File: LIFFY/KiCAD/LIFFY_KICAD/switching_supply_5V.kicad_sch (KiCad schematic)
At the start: 6 parts, among them U7 AP63205WU

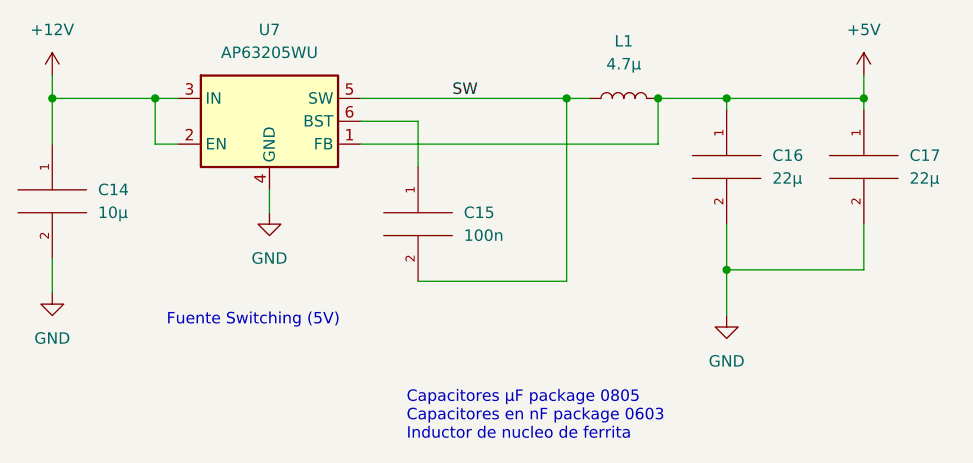
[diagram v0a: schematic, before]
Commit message: V3 Fixed
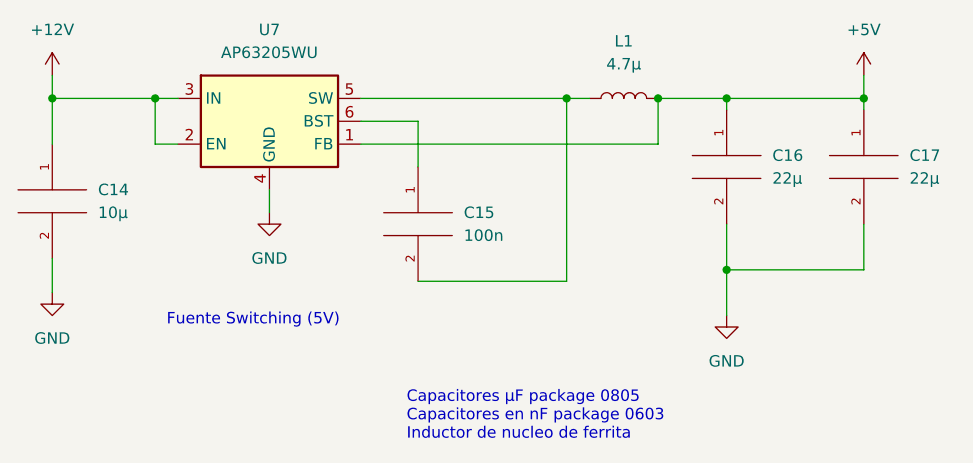
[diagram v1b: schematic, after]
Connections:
- net SW: no longer names the net of C15.2, L1.1, U7.5 (SW)
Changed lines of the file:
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@@
-    (effects (font (size 1.27 1.27)) (justify left bottom))
-  )
-  (label "SW" (at 146.05 91.44 0)
     (effects (font (size 1.27 1.27)) (justify left bottom))
   )

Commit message: V4.5 Fixed
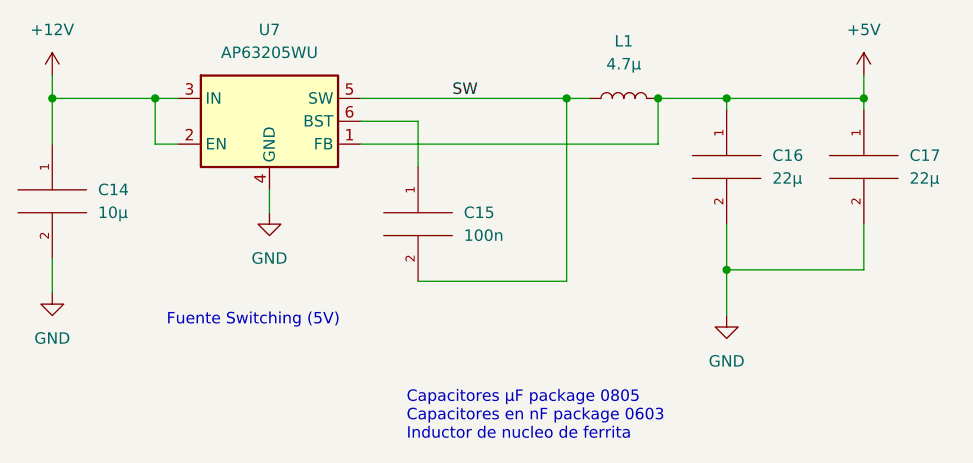
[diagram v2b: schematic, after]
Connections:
- net SW: now reaches C15.2, L1.1, U7.5 (SW)
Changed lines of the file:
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@@
+    (effects (font (size 1.27 1.27)) (justify left bottom))
+  )
+  (label "SW" (at 146.05 91.44 0)
     (effects (font (size 1.27 1.27)) (justify left bottom))
   )
